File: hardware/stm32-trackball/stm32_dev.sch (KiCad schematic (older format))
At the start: 60 parts, among them J1 USB_C_Receptacle_USB2.0, J2 SWD, J3 UART, J4 SPARE, J5 Breakout, J6 Breakout, SW1 KMR2, SW2 KMR2, SW3 SW_Push, SW4 KMR2, SW5 KMR2, SW6 KMR2, T1 Trackball, U1 AP2112K-3.3, U2 USBLC6-2SC6, U3 STM32F042G6Ux, U4 AN48840B, U5 AN48840B, U6 AN48840B, U7 AN48840B

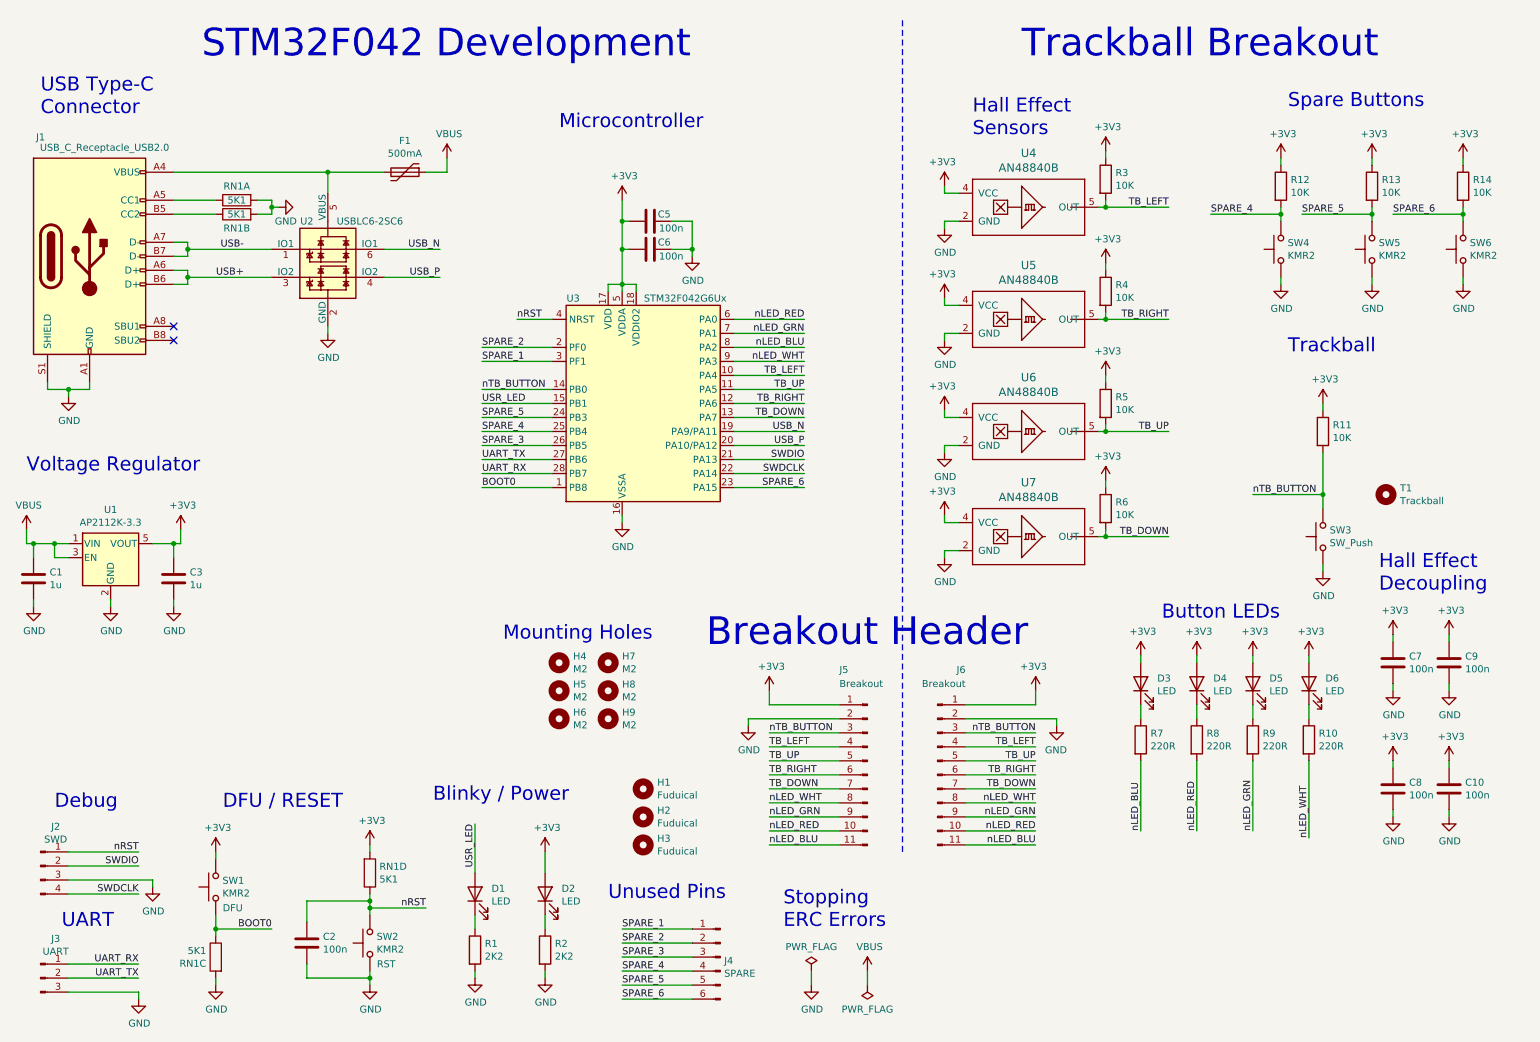
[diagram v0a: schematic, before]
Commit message: 2u layout somehow passes DRC
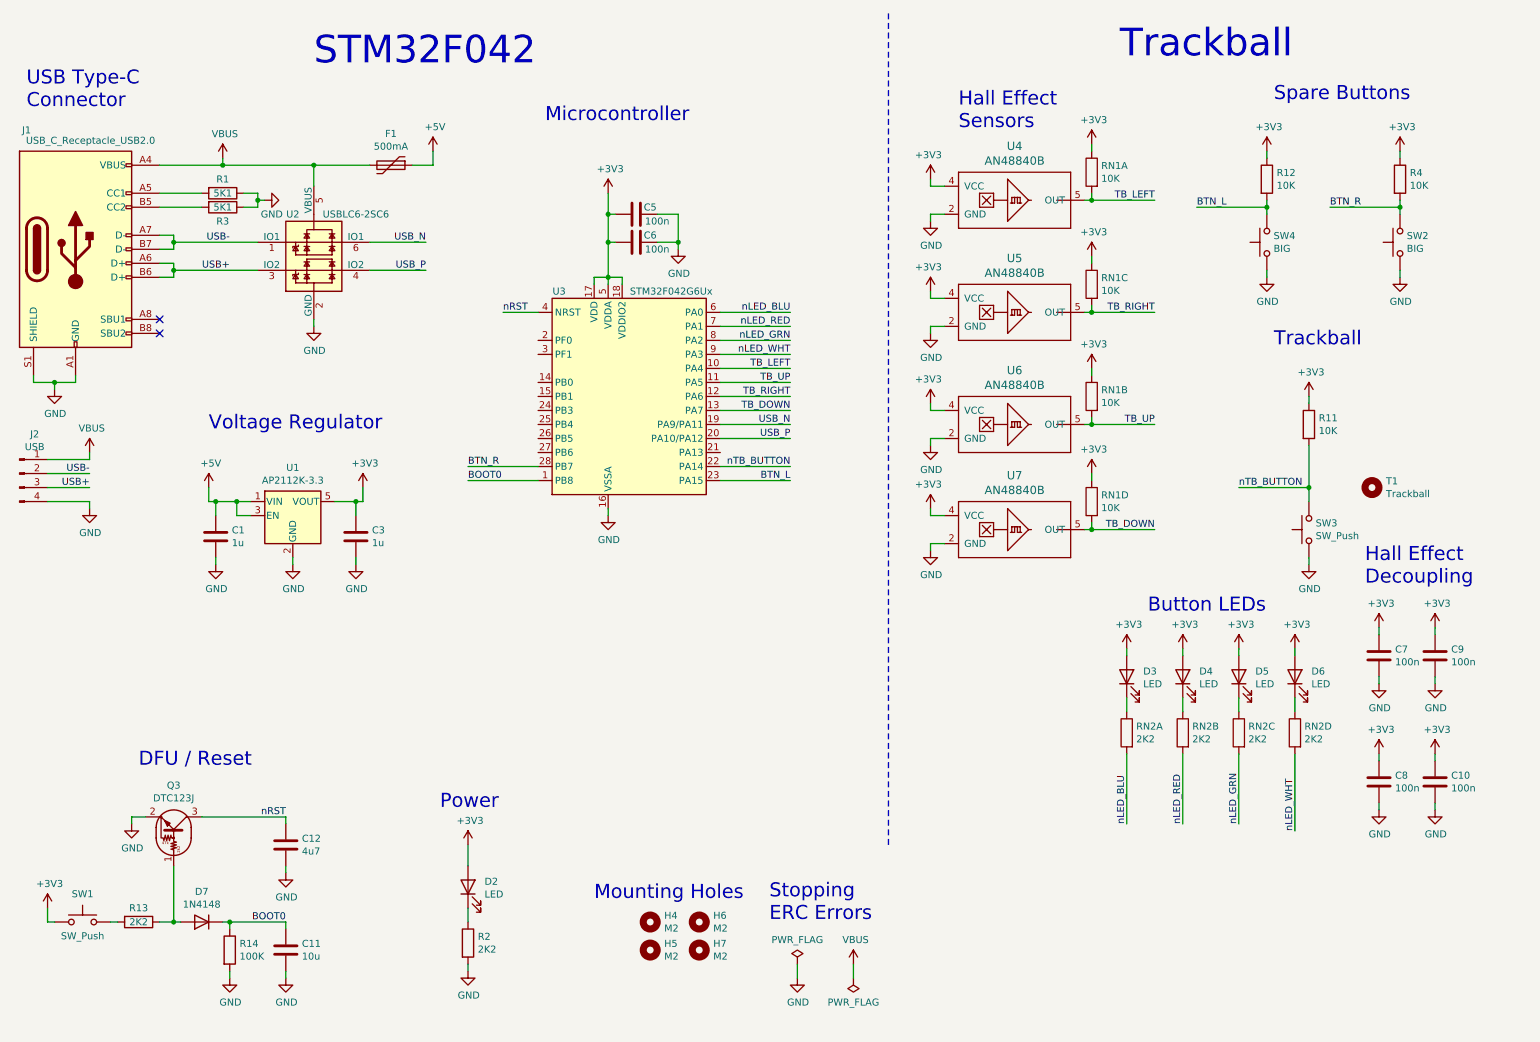
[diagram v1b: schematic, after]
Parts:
- removed C2: 100n, Capacitor_SMD:C_0603_1608Metric, symbol Device:C
- removed D1: LED, LED_SMD:LED_0603_1608Metric, symbol Device:LED
- removed H1, H2, H3: Fuduical, Fiducial:Fiducial_1mm_Mask2mm, symbol Mechanical:MountingHole
- removed H8, H9: M2, MountingHole:MountingHole_2.2mm_M2, symbol Mechanical:MountingHole
- removed J3: UART, josh-connectors:STM_3_PIN_THT_Staggered, symbol Connector:Conn_01x03_Male
- removed J4: SPARE, Connector_PinHeader_2.54mm:PinHeader_1x06_P2.54mm_Vertical, symbol Connector:Conn_01x06_Male
- removed J5, J6: Breakout, Connector_PinHeader_2.54mm:PinHeader_1x11_P2.54mm_Vertical, symbol Connector:Conn_01x11_Male
- removed R10, R7, R8, R9: 220R, Resistor_SMD:R_0603_1608Metric, symbol Device:R
- removed R5, R6: 10K, Resistor_SMD:R_0603_1608Metric, symbol Device:R
- removed SW5, SW6: KMR2, josh-buttons-switches:SW_Push_KMR2, symbol Switch:SW_Push
- added C11: 10u, Capacitor_SMD:C_0402_1005Metric, symbol Device:C
- added C12: 4u7, Capacitor_SMD:C_0402_1005Metric, symbol Device:C
- added D7: 1N4148, Diode_SMD:D_SOD-323, symbol Device:D
- added Q3: DTC123J, Package_TO_SOT_SMD:SOT-23, symbol Transistor_BJT:DTC123J
- added RN2: 2K2, Resistor_SMD:R_Array_Convex_4x0402, symbol josh-passive:RN
- C1, C10, C3, C5, C6, C7, C8, C9: footprint Capacitor_SMD:C_0603_1608Metric -> Capacitor_SMD:C_0402_1005Metric
- J2: value SWD -> USB; footprint josh-connectors:STM_4_PIN_THT_Staggered -> Connector_PinHeader_1.27mm:PinHeader_1x04_P1.27mm_Vertical
- R1: value 2K2 -> 5K1; footprint Resistor_SMD:R_0603_1608Metric -> Resistor_SMD:R_0402_1005Metric; JLCSMT (none) -> C22843; LCSC (none) -> C22843; MPN (none) -> 0603WAF1501T5E; Manufacturer (none) -> Uniroyal Elec
- R11, R12, R2, R4: footprint Resistor_SMD:R_0603_1608Metric -> Resistor_SMD:R_0402_1005Metric
- R13: value 10K -> 2K2; footprint Resistor_SMD:R_0603_1608Metric -> Resistor_SMD:R_0402_1005Metric; JLCSMT (none) -> C22843; LCSC (none) -> C22843; MPN (none) -> 0603WAF1501T5E; Manufacturer (none) -> Uniroyal Elec
- R14: value 10K -> 100K; footprint Resistor_SMD:R_0603_1608Metric -> Resistor_SMD:R_0402_1005Metric; JLCSMT (none) -> C25803; LCSC (none) -> C25803; MPN (none) -> 0603WAF1003T5E; Manufacturer (none) -> Uniroyal Elec
- R3: value 10K -> 5K1; footprint Resistor_SMD:R_0603_1608Metric -> Resistor_SMD:R_0402_1005Metric; JLCSMT (none) -> C22843; LCSC (none) -> C22843; MPN (none) -> 0603WAF1501T5E; Manufacturer (none) -> Uniroyal Elec
- RN1: value 5K1 -> 10K; footprint Resistor_SMD:R_Array_Convex_4x0603 -> Resistor_SMD:R_Array_Convex_4x0402; DigiKey CAY16-512J4LFCT-ND -> (none); LCSC C12028 -> (none); MPN CAY16-512J4LF -> (none); Manufacturer Bourns -> (none); Notes LCSC PN Sub -> (none)
- SW1: value KMR2 -> SW_Push; footprint josh-buttons-switches:SW_Push_KMR2 -> josh-buttons-switches:Panasonic_EVQPUL_EVQPUC; DigiKey CKN10884CT-ND -> (none); LCSC C221909 -> (none); MPN PTS840GMSMTRLFS -> (none); Manufacturer C&K -> (none); Name DFU -> (none); Notes Substutite okay -> (none)
- SW2: value KMR2 -> BIG; footprint josh-buttons-switches:SW_Push_KMR2 -> josh-buttons-switches:Switch_SMT_SKPMAPE010; DigiKey CKN10884CT-ND -> (none); LCSC C221909 -> (none); MPN PTS840GMSMTRLFS -> (none); Manufacturer C&K -> (none); Name RST -> (none); Notes Substutite okay -> (none)
- SW4: value KMR2 -> BIG; footprint josh-buttons-switches:SW_Push_KMR2 -> josh-buttons-switches:Switch_SMT_SKPMAPE010; DigiKey CKN10884CT-ND -> (none); LCSC C221909 -> (none); MPN PTS840GMSMTRLFS -> (none); Manufacturer C&K -> (none); Notes Substutite okay -> (none)
- U2: footprint Package_TO_SOT_SMD:SOT-23-6 -> Package_TO_SOT_SMD:SOT-666
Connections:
- net +3V3: now also RN1.5, RN1.6, RN1.7, RN1.8, SW1.1; no longer R13.1, R14.1, R3.1, RN1.1, SW1.2
- net BOOT0: now also R14.1, C11.1, D7.1 (K); no longer RN1.7, SW1.1
- net GND: now also J2.4 (Pin_4), R1.1, R14.2, R3.1, C11.2, C12.2, Q3.2 (E); no longer J2.3 (Pin_3), R1.2, RN1.2, RN1.3, RN1.4
- net TB_DOWN: now also RN1.1
- net TB_LEFT: now also RN1.4; no longer R3.2
- net TB_RIGHT: now also RN1.2; no longer R4.2
- net TB_UP: now also RN1.3
- net USB+: now also J2.3 (Pin_3)
- net USB-: now also J2.2 (Pin_2)
- net VBUS: now also F1.2, J1.A4 (VBUS), J1.A9 (VBUS), J1.B4 (VBUS), J1.B9 (VBUS), J2.1 (Pin_1), U2.5 (VBUS); no longer C1.2, F1.1, U1.1 (VIN), U1.3 (EN)
- net nLED_BLU: now also U3.6 (PA0), RN2.4; no longer U3.8 (PA2)
- net nLED_GRN: now also U3.8 (PA2), RN2.2; no longer U3.7 (PA1)
- net nLED_RED: now also U3.7 (PA1), RN2.3; no longer U3.6 (PA0)
- net nLED_WHT: now also RN2.1
- net nRST: now also C12.1, Q3.3 (C); no longer J2.1 (Pin_1), RN1.8, SW2.2
- net nTB_BUTTON: now also U3.22 (PA14); no longer U3.14 (PB0)
- net at J1.A5 (CC1): now also R1.2; no longer RN1.5
- net at J1.B5 (CC2): now also R3.2; no longer RN1.6
- net at D6.1 (K): now also RN2.8
- net at D5.1 (K): now also RN2.7
- net at D4.1 (K): now also RN2.6
- net at D3.1 (K): now also RN2.5
- net SPARE_1: no longer names the net of U3.3 (PF1)
- net SPARE_2: no longer names the net of U3.2 (PF0)
- net SPARE_3: no longer names the net of U3.26 (PB5)
- net SPARE_4 renamed BTN_L
- net BTN_L: now also U3.23 (PA15); no longer U3.25 (PB4)
- net SPARE_5: no longer names the net of U3.24 (PB3)
- net SPARE_5: no longer R13.2
- removed net SPARE_6: R14.2, U3.23 (PA15)
- removed net SWDCLK: J2.4 (Pin_4), U3.22 (PA14)
- net SWDIO: no longer names the net of U3.21 (PA13)
- net SWDIO: no longer J2.2 (Pin_2)
- net UART_RX renamed BTN_R
- net BTN_R: now also R4.2, SW2.2
- net UART_TX: no longer names the net of U3.27 (PB6)
- net USR_LED: no longer names the net of U3.15 (PB1)
- new net: D7.2 (A), Q3.1 (B), R13.1
- new net: R13.2, SW1.2
- new net +5V: C1.2, F1.1, U1.1 (VIN), U1.3 (EN)
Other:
- note added: "DFU / Reset"
- note added: "Power"
- note added: "STM32F042"
- note removed: "Blinky / Power"
- note removed: "Breakout Header"
- note removed: "DFU / RESET"
- note removed: "Debug"
- note removed: "STM32F042 Development"
- note removed: "Trackball Breakout"
- note removed: "UART"
- note removed: "Unused Pins"
- moved on the sheet: C1, C10, C3, C5, C6, C7, C8, C9, D2, D3, D4, D5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
